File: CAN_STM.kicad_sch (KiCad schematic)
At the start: 1 part, among them IC2 TCAN3414DRBR

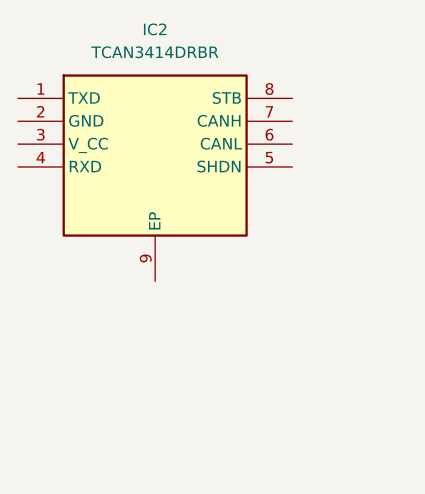
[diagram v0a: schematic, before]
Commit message: can
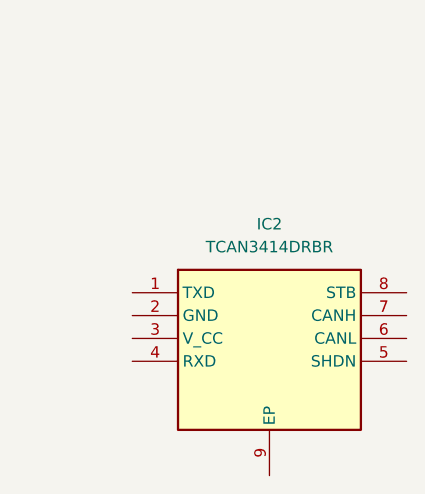
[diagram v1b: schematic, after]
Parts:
- IC2: footprint dz_comm_TCAN3414DRBR -> dz_comm:TCAN3414DRBR
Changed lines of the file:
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@@
 	(symbol
 		(lib_id "#dzdb:s_comm/COMM-TI-TCAN3414DRBR")
-		(at 106.68 77.47 0)
+		(at 119.38 99.06 0)
 		(unit 1)
 		(exclude_from_sim no)
@@
 		(fields_autoplaced yes)
 		(property "Reference" "IC2"
-			(at 121.92 69.85 0)
+			(at 134.62 91.44 0)
 			(effects
 				(font
@@
 		)
 		(property "Value" "TCAN3414DRBR"
-			(at 121.92 72.39 0)
-			(effects
-				(font
-					(size 1.27 1.27)
-				)
-			)
-		)
-		(property "Footprint" "dz_comm_TCAN3414DRBR"
-			(at 133.35 172.39 0)
+			(at 134.62 93.98 0)
+			(effects
+				(font
+					(size 1.27 1.27)
+				)
+			)
+		)
+		(property "Footprint" "dz_comm:TCAN3414DRBR"
+			(at 146.05 193.98 0)
 			(effects
 				(font
@@
 		)
 		(property "Datasheet" "https://www.ti.com/lit/gpn/tcan3414"
-			(at 133.35 272.39 0)
+			(at 146.05 293.98 0)
 			(effects
 				(font
@@
 		)
 		(property "Description" "CAN Interface IC CAN FD Transceiver with Integrated Controller"
-			(at 106.68 77.47 0)
+			(at 119.38 99.06 0)
 			(effects
 				(font
@@
 		)
 		(property "Height" "1"
-			(at 133.35 472.39 0)
+			(at 146.05 493.98 0)
 			(effects
 				(font
@@
 		)
 		(property "Mouser Part Number" "595-TCAN3414DRBR"
-			(at 133.35 572.39 0)
+			(at 146.05 593.98 0)
 			(effects
 				(font
@@
 		)
 		(property "Mouser Price/Stock" "https://www.mouser.co.uk/ProductDetail/Texas-Instruments/TCAN3414DRBR?qs=2wMNvWM5ZX6YBBH9qF6w4g%3D%3D"
-			(at 133.35 672.39 0)
+			(at 146.05 693.98 0)
 			(effects
 				(font
@@
 		)
 		(property "Manufacturer_Name" "Texas Instruments"
-			(at 133.35 772.39 0)
+			(at 146.05 793.98 0)
 			(effects
 				(font
@@
 		)
 		(property "Manufacturer_Part_Number" "TCAN3414DRBR"
-			(at 133.35 872.39 0)
+			(at 146.05 893.98 0)
 			(effects
 				(font
@@
 		)
 		(property "IPN" "COMM-TI-TCAN3414DRBR"
-			(at 106.68 77.47 0)
+			(at 119.38 99.06 0)
 			(effects
 				(font
@@
 		)
 		(property "MPN" "TCAN3414DRBR"
-			(at 106.68 77.47 0)
+			(at 119.38 99.06 0)
 			(effects
 				(font
@@
 		)
 		(property "Manufacturer" "Texas Instruments"
-			(at 106.68 77.47 0)
+			(at 119.38 99.06 0)
 			(effects
 				(font
@@
 		)
 		(property "Type" "Can Tranciever"
-			(at 106.68 77.47 0)
+			(at 119.38 99.06 0)
 			(effects
 				(font
@@
 		)
 		(property "Supply" "3V-3.3V"
-			(at 106.68 77.47 0)
+			(at 119.38 99.06 0)
 			(effects
 				(font
@@
 		)
 		(property "Package" "SON-8"
-			(at 106.68 77.47 0)
+			(at 119.38 99.06 0)
 			(effects
 				(font
@@
 		)
 		(property "Supplier" "Mouser"
-			(at 106.68 77.47 0)
+			(at 119.38 99.06 0)
 			(effects
 				(font
@@
 		)
 		(property "SPN" " 595-TCAN3414DRBR"
-			(at 106.68 77.47 0)
+			(at 119.38 99.06 0)
 			(effects
 				(font
@@
 		)
 		(property "LCSC" "Cxxxxxx"
-			(at 106.68 77.47 0)
+			(at 119.38 99.06 0)
 			(effects
 				(font
@@
 		)
 		(property "Comment" ""
-			(at 106.68 77.47 0)
-			(effects
-				(font
-					(size 1.27 1.27)
-				)
-				(hide yes)
-			)
+			(at 119.38 99.06 0)
+			(effects
+				(font
+					(size 1.27 1.27)
+				)
+				(hide yes)
+			)
+		)
+		(pin "9"
+		)
+		(pin "7"
+		)
+		(pin "4"
+		)
+		(pin "6"
+		)
+		(pin "5"
+		)
+		(pin "3"
+		)
+		(pin "8"
 		)
 		(pin "1"
 		)
 		(pin "2"
-		)
-		(pin "3"
-		)
-		(pin "4"
-		)
-		(pin "8"
-		)
-		(pin "7"
-		)
-		(pin "6"
-		)
-		(pin "5"
-		)
-		(pin "9"
 		)
 		(instances
 			(project ""
-				(path "/ce1819b2-f280-40ed-834f-6fe4d12f809d/46fb4fb5-44f2-465b-b1ff-e4e0fbef74ae/b861b505-f377-49fb-9e06-1714af927ea6"
+				(path "/ce1819b2-f280-40ed-834f-6fe4d12f809d/46fb4fb5-44f2-465b-b1ff-e4e0fbef74ae/58617765-d176-459f-be30-726b62920b6c"
 					(reference "IC2")
 					(unit 1)
